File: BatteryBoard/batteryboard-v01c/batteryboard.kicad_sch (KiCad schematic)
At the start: 36 parts, among them J1 KEYSTONE-1042, J2 KEYSTONE-1042, J3 KEYSTONE-1042, J4 KEYSTONE-1042, J5 KEYSTONE-1042, J6 KEYSTONE-1042, J7 MOLEX 5023520801, J8 Screw_Terminal_01x02, Q1 IRF7458, Q2 IRF7458, Q3 IRLML2803, Q4 IRLML2803, Q5 IRF7404TRPBF, U1 R5460N233AF

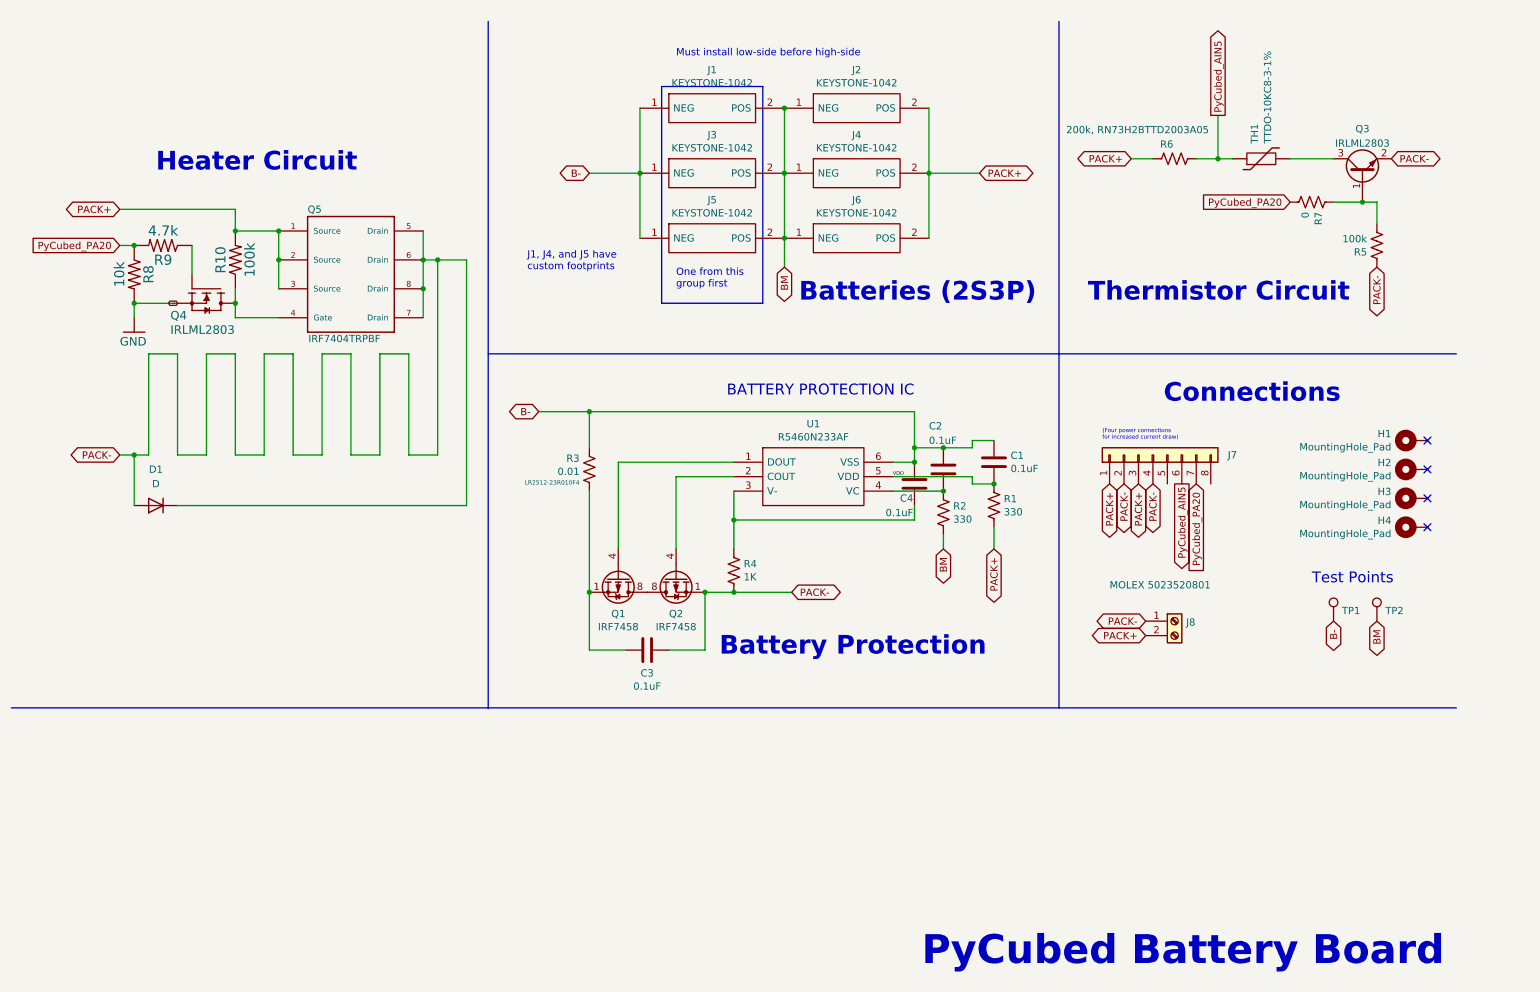
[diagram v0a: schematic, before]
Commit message: Updated PCB
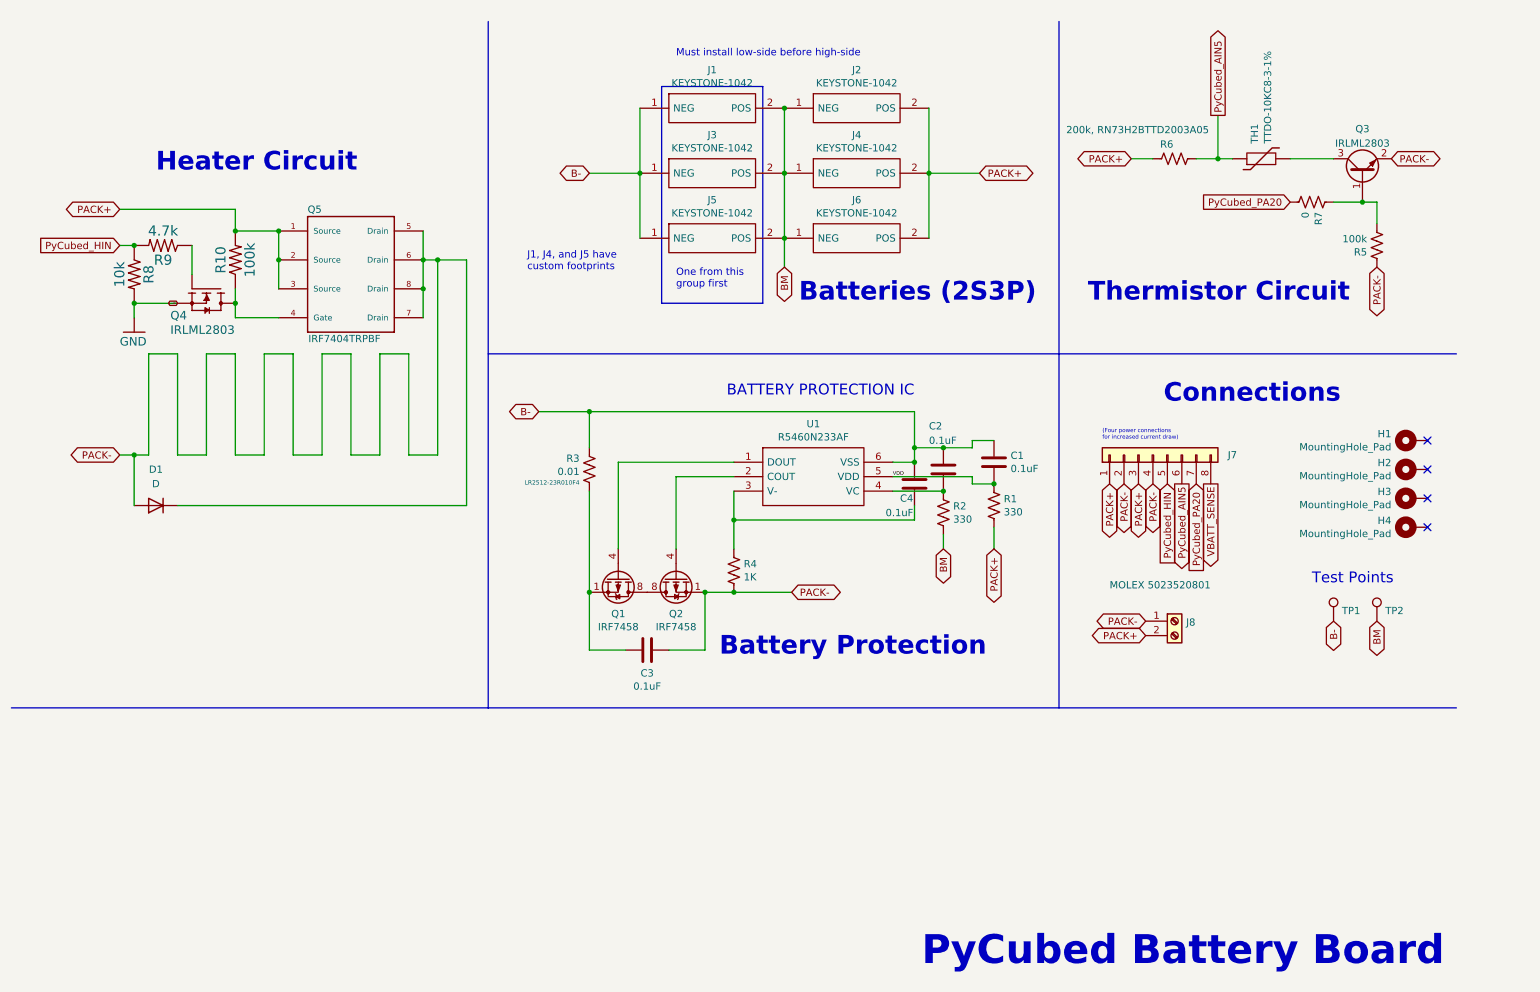
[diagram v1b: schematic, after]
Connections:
- net PyCubed_PA20: no longer R8.1, R9.2
- net PyCubed_HIN: now reaches J7.5 (Pin_5)
- net PyCubed_HIN: now also R8.1, R9.2
- net VBATT_SENSE: now reaches J7.8 (Pin_8)
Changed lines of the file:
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@@
   (global_label "PyCubed_AIN5" (shape output) (at 218.44 95.25 270) (fields_autoplaced)
     (effects (font (size 1.27 1.27)) (justify right))
-    (property "Intersheetrefs" "${INTERSHEET_REFS}" (at 218.44 110.7458 90)
+    (property "Intersheetrefs" "${INTERSHEET_REFS}" (at 218.44 110.8252 90)
+      (effects (font (size 1.27 1.27)) (justify right) hide)
+    )
+  )
+  (global_label "PyCubed_HIN" (shape input) (at 215.9 95.25 270) (fields_autoplaced)
+    (effects (font (size 1.27 1.27)) (justify right))
+    (property "Intersheetrefs" "${INTERSHEET_REFS}" (at 215.9 109.8576 90)
       (effects (font (size 1.27 1.27)) (justify right) hide)
     )
@@
     (effects (font (size 1.27 1.27)) (justify right))
     (property "Intersheetrefs" "${INTERSHEET_REFS}" (at 221.45 45.72 0)
-      (effects (font (size 1.27 1.27)) (justify right) hide)
-    )
-  )
-  (global_label "PyCubed_PA20" (shape input) (at 31.75 53.34 180) (fields_autoplaced)
-    (effects (font (size 1.27 1.27)) (justify right))
-    (property "Intersheetrefs" "${INTERSHEET_REFS}" (at 15.6306 53.34 0)
       (effects (font (size 1.27 1.27)) (justify right) hide)
     )
@@
     )
   )
+  (global_label "PyCubed_HIN" (shape input) (at 31.75 53.34 180) (fields_autoplaced)
+    (effects (font (size 1.27 1.27)) (justify right))
+    (property "Intersheetrefs" "${INTERSHEET_REFS}" (at 17.1424 53.34 0)
+      (effects (font (size 1.27 1.27)) (justify right) hide)
+    )
+  )
   (global_label "PACK+" (shape bidirectional) (at 205.74 95.25 270) (fields_autoplaced)
     (effects (font (size 1.27 1.27)) (justify right))
@@
       (effects (font (size 1.27 1.27)) (justify right) hide)
     )
+  )
+  (global_label "VBATT_SENSE" (shape output) (at 223.52 95.25 270) (fields_autoplaced)
+    (effects (font (size 1.27 1.27)) (justify right))
+    (property "Intersheetrefs" "${INTERSHEET_REFS}" (at 223.52 109.9785 90)
+      (effects (font (size 1.27 1.27)) (justify right) hide)
+    )
